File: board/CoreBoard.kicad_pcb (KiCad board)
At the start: 2 copper layers, 121.9 x 87.4 mm, 94 parts, among them J1 RJ45_LED_Shielded, J2 768250002, Q1 AO3401A, Q10 AO3401A, Q11 AO3401A, Q2 AO3401A, Q3 AO3401A, Q4 AO3401A, Q5 AO3401A, Q6 AO3401A, Q7 AO3401A, Q8 AO3401A, Q9 AO3401A, SW11 SW_Wuerth_450301014042, SW12 SW_Wuerth_450301014042, SW13 SW_Wuerth_450301014042, SW14 SW_Wuerth_450301014042, SW15 SW_Wuerth_450301014042, SW16 SW_Wuerth_450301014042, SW4 SW_Push, SW6 SW_Push, SW7 SW_Push, SW8 SW_Push, U1 74VHC138FT, U2 OKI-78SR-12_1.0-W36H-C, U3 SHHD003A0A, U4 GY-521, U5 Teensy4.1_DEV-16771, U6 MCP9808-E/MS

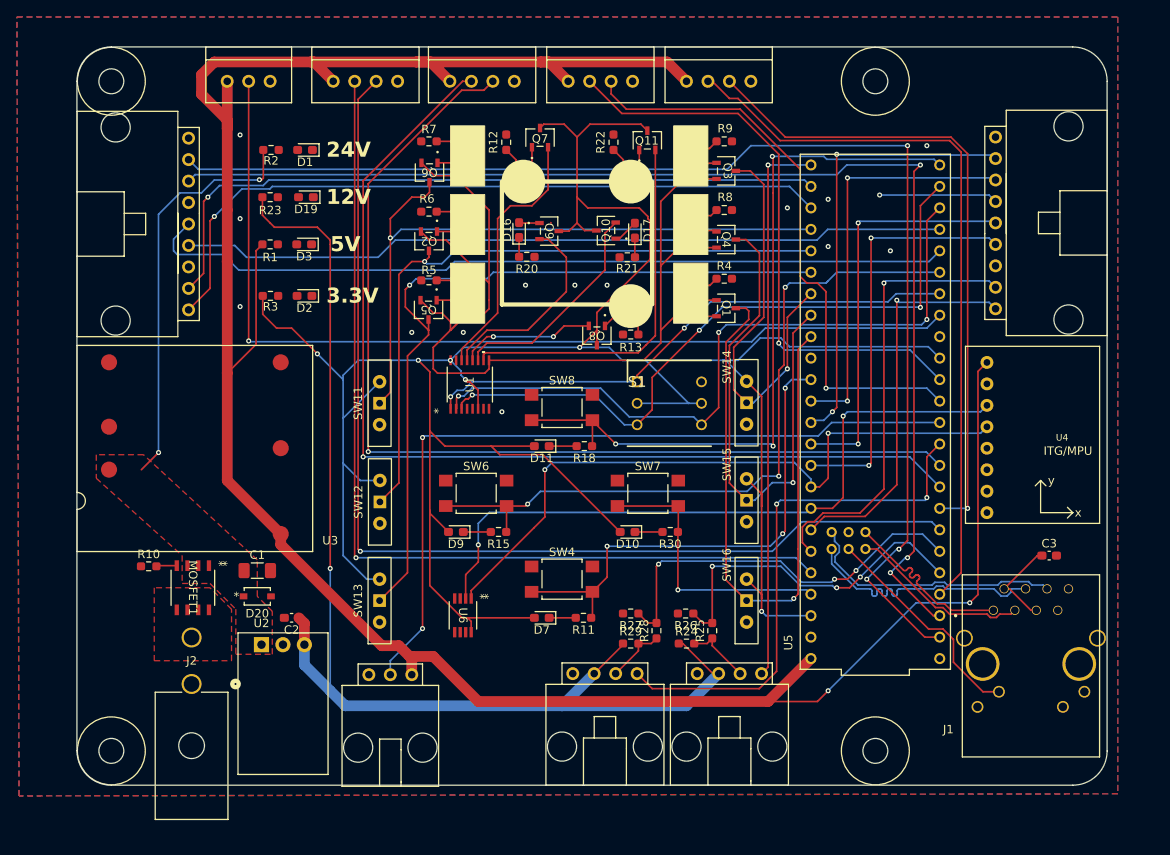
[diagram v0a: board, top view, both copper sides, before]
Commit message: route
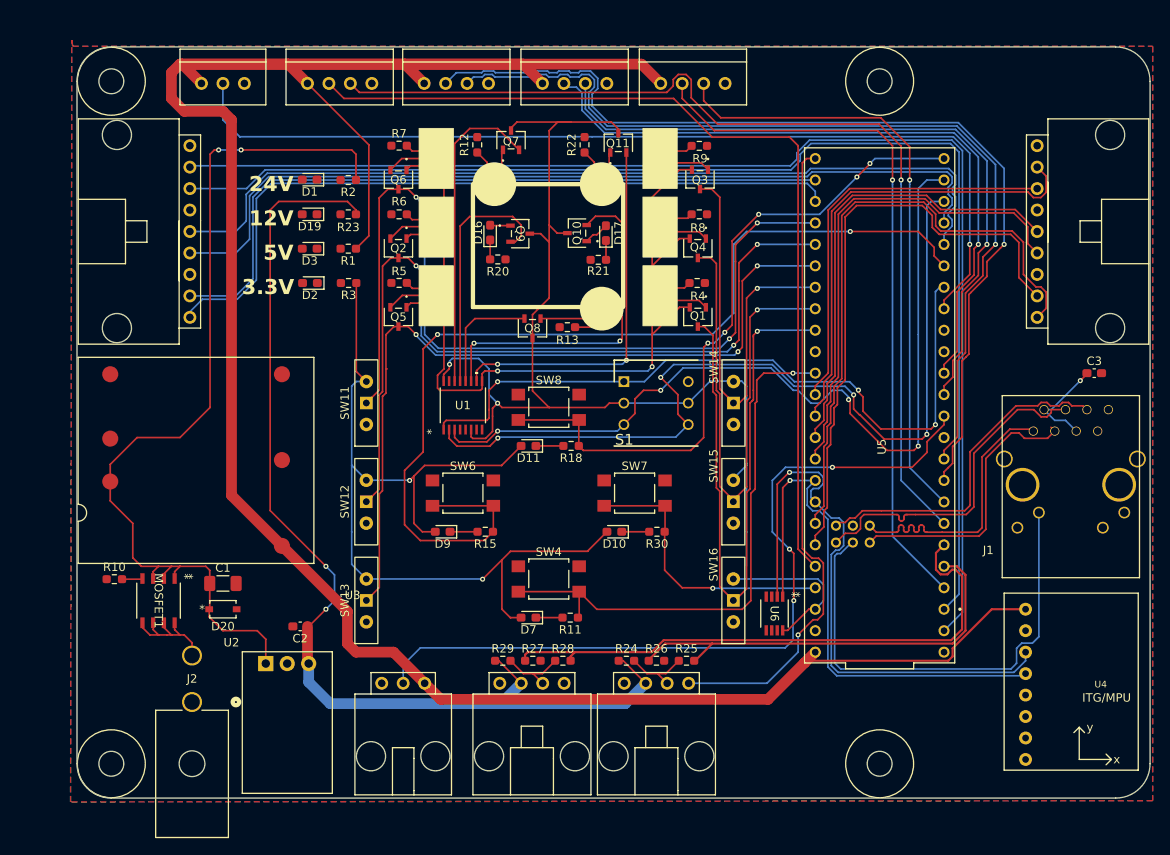
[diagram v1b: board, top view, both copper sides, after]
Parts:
- moved U6 36.9 mm to (155.7, 117.9)
- moved U4 29.6 mm to (194.3, 126.2)
- moved C3 22.2 mm to (193.5, 89.4)
- moved J1 21.7 mm to (190.9, 115.6)
- moved R29 15.3 mm to (123.5, 123.4)
- moved R27 12.9 mm to (127.1, 123.4), turned to 0 degrees
- moved R28 11.6 mm to (130.7, 123.4), turned to 0 degrees
- moved R2 9.81 mm to (105.3, 66.5), turned to 180 degrees
- moved R23 9.46 mm to (105.3, 70.6), turned to 180 degrees
- moved R3 9.37 mm to (105.3, 78.7), turned to 180 degrees
- moved R1 9.26 mm to (105.3, 74.7), turned to 180 degrees
- moved Conn2 8.71 mm to (145.5, 126.1)
- moved Conn9 8.71 mm to (130.8, 126.1)
- moved Q8 7.67 mm to (127.1, 84.1)
- moved R13 7.54 mm to (131.2, 84.0)
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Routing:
- net +3.3V: track 336.5 -> 259.2 mm, vias 6 -> 4
- net /Fans/PWM2: track 63.0 -> 0.00 mm, vias 2 -> 0
- net VCC: track 48.6 -> 108.6 mm
- net /Teensy/Left: track 86.0 -> 118.1 mm, vias 3 -> 2
- net LED: track 26.4 -> 57.6 mm
- net /Motor VESCs/BR_TX: track 46.3 -> 73.5 mm, vias 1 -> 0
- net /Selection LEDs/FL_EN: track 79.7 -> 105.9 mm, vias 1 -> 3
- net /Fans/Tach2: track 47.3 -> 68.4 mm, vias 3 -> 0
- net /Selection LEDs/RTRY4: track 80.1 -> 101.2 mm, vias 3 -> 4
- net /Selection LEDs/RTRY1: track 64.8 -> 85.7 mm, vias 2 -> 3
- net /Selection LEDs/RTRY2: track 83.5 -> 104.2 mm, vias 3 -> 4
- net /Selection LEDs/ML_EN: track 79.5 -> 100.0 mm, vias 1 -> 3
- net /Motor VESCs/BR_RX: track 52.8 -> 71.2 mm, vias 1 -> 0
- net +5V: track 286.5 -> 304.7 mm, vias 2 -> 0
- net /Selection LEDs/Spare2: track 26.2 -> 41.0 mm, vias 0 -> 2
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- removed copper zone on F.Cu, net Net-(J2-Pad2)
- removed copper zone on F.Cu, net VCC
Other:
- board size 121.9 x 87.4 mm -> 127 x 88.9 mm

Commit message: Update CoreBoard.kicad_pcb
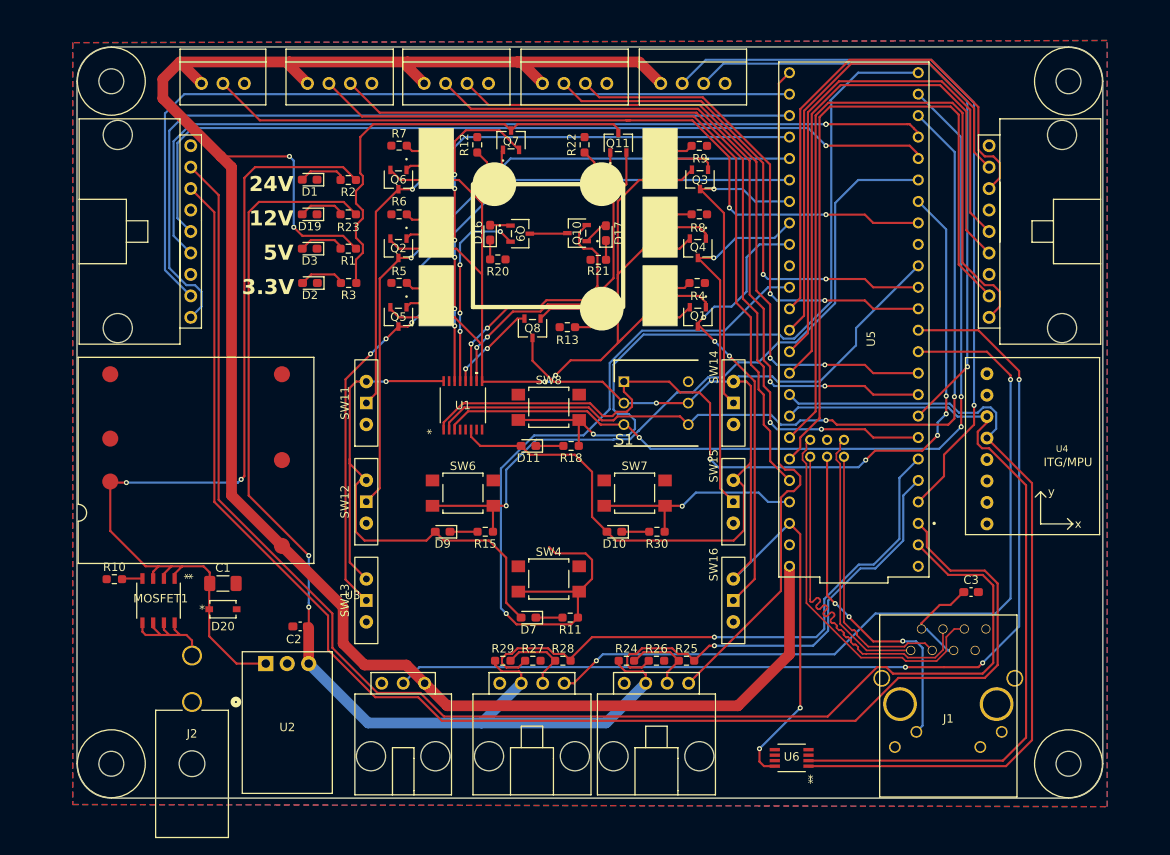
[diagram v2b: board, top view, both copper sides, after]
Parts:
- moved J1 29.7 mm to (176.4, 141.6)
- moved C3 29.7 mm to (179.0, 115.3)
- moved U4 28.2 mm to (189.7, 98.4)
- moved H1 22.4 mm to (190.5, 54.9)
- moved H4 22.4 mm to (190.5, 135.6)
- moved U6 17.2 mm to (157.7, 134.9), turned to 180 degrees
- moved U5 10.6 mm to (165.1, 83.1)
- moved Conn4 5.69 mm to (181.1, 62.5)
- moved Conn3 0.10 mm to (86.6, 82.8)
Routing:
- net /Fans/PWM2: track 0.00 -> 95.5 mm, vias 0 -> 2
- net +5V: track 304.7 -> 244.9 mm, vias 0 -> 2
- net +3.3V: track 259.2 -> 308.1 mm
- net /Teensy/Left: track 118.1 -> 86.1 mm, vias 2 -> 1
- net /Selection LEDs/FL_EN: track 105.9 -> 75.7 mm, vias 3 -> 1
- net /Accelerometer/AccSDA: track 65.0 -> 95.0 mm, vias 1 -> 0
- net /Gimbal Servos/LeftPan: track 114.7 -> 85.1 mm, vias 1 -> 2
- net /Gimbal Servos/LeftTilt: track 108.4 -> 80.3 mm, vias 1 -> 2
- net /Teensy/Back: track 65.6 -> 93.5 mm
- net /Lighting/Lighting_Panel: track 94.3 -> 119.9 mm
- net /Gimbal Servos/BackTilt: track 82.9 -> 59.4 mm, vias 1 -> 2
- net /Accelerometer/AccSCL: track 70.8 -> 92.4 mm, vias 1 -> 0
- net /Gimbal Servos/BackPan: track 81.1 -> 59.7 mm, vias 1 -> 2
- net /Motor VESCs/FL_TX: track 148.9 -> 169.8 mm
- net /Selection LEDs/BR_EN: track 74.7 -> 53.9 mm, vias 1 -> 3
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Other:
- board size 127 x 88.9 mm -> 121.4 x 88.9 mm
